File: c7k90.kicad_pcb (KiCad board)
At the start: 2 copper layers, 71.5 x 27.1 mm, 5 parts, among them J1 Conn_01x02_Socket, J2 Conn_01x04_Socket, J3 Conn_01x04_Pin, SW1 SW_SPST, U1 Nice! Nano (ProMicro)

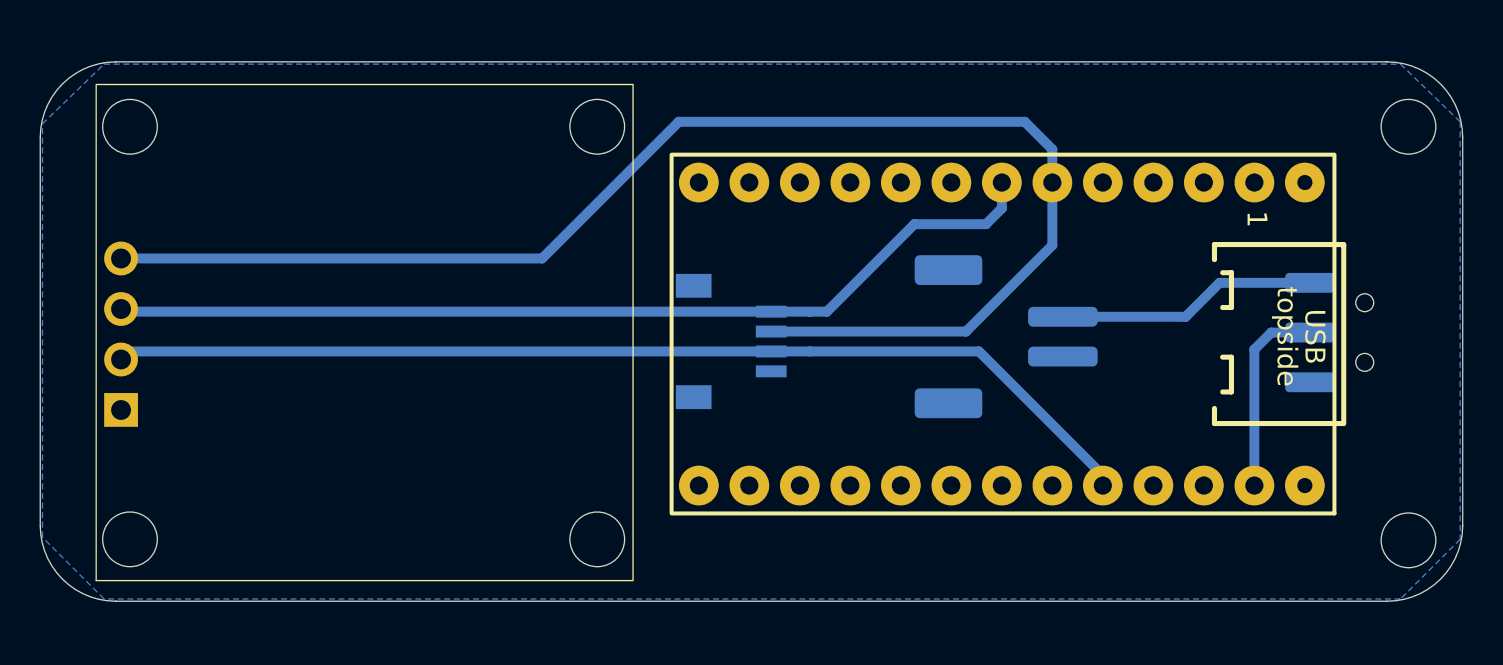
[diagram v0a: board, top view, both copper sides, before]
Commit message: updates
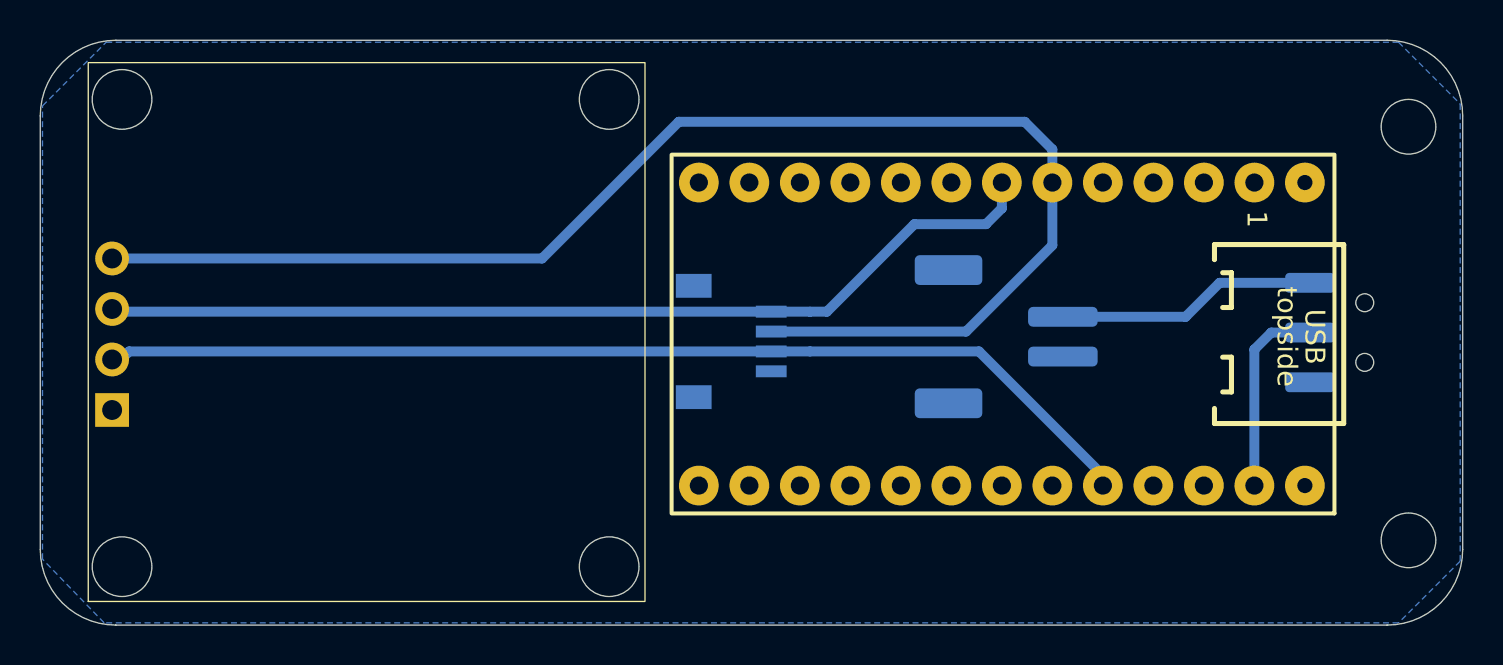
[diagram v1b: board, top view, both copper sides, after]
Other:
- board size 71.5 x 27.1 mm -> 71.5 x 29.4 mm
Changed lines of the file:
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@@
 		(attr through_hole)
 		(fp_rect
-			(start -12.45 -12)
-			(end 12.5 15)
+			(start -13.5 -12.4)
+			(end 13.6 15.6)
 			(stroke
 				(width 0.05)
@@
 		)
 		(fp_circle
-			(center 10.375 -10.3)
-			(end 10.375 -11.675)
+			(center 11.75 -10.7)
+			(end 13.25 -10.7)
 			(stroke
 				(width 0.05)
@@
 		)
 		(fp_circle
-			(center -10.375 -10.3)
-			(end -10.375 -11.675)
+			(center -11.75 -10.7)
+			(end -10.25 -10.7)
 			(stroke
 				(width 0.05)
@@
 		)
 		(fp_circle
-			(center 10.375 13.2)
-			(end 11.75 13.2)
+			(center 11.75 13.8)
+			(end 13.25 13.8)
 			(stroke
 				(width 0.05)
@@
 		)
 		(fp_circle
-			(center -10.375 13.2)
-			(end -9 13.2)
+			(center -11.75 13.8)
+			(end -10.25 13.8)
 			(stroke
 				(width 0.05)
@@
 		)
 		(pad "1" thru_hole rect
-			(at -3.87 -10.75 90)
+			(at -3.87 -11.2 90)
 			(size 1.7 1.7)
 			(drill 1)
@@
 		)
 		(pad "2" thru_hole circle
-			(at -1.33 -10.75 90)
+			(at -1.33 -11.2 90)
 			(size 1.7 1.7)
 			(drill 1)
@@
 		)
 		(pad "3" thru_hole circle
-			(at 1.21 -10.75 90)
+			(at 1.21 -11.2 90)
 			(size 1.7 1.7)
 			(drill 1)
@@
 		)
 		(pad "4" thru_hole circle
-			(at 3.75 -10.75 90)
+			(at 3.75 -11.2 90)
 			(size 1.7 1.7)
 			(drill 1)
@@
 		)
 		(embedded_fonts no)
-		(model "/Users/sklarm/Documents/KiCad/mikeysklar/3dmodels/oled-ssd1306.step"
+		(model "/Users/sklarm/Documents/KiCad/mikeysklar/3dmodels/blue-oled-ssd1306-128x64.step"
 			(offset
-				(xyz 0 -1 0)
+				(xyz 0 -1.5 0)
 			)
 			(scale
@@
 	)
 	(gr_line
-		(start 209.125988 72.987007)
-		(end 145.187006 72.987006)
+		(start 209.125988 71.900001)
+		(end 145.187006 71.9)
 		(stroke
 			(width 0.05)
@@
 	)
 	(gr_arc
-		(start 212.925988 96.312994)
-		(mid 211.812994 99)
-		(end 209.125988 100.112994)
+		(start 212.925988 97.512994)
+		(mid 211.812994 100.2)
+		(end 209.125988 101.312994)
 		(stroke
 			(width 0.05)
@@
 	)
 	(gr_arc
-		(start 209.125988 72.987006)
-		(mid 211.812994 74.1)
-		(end 212.925988 76.787006)
+		(start 209.125988 71.9)
+		(mid 211.812999 73.01299)
+		(end 212.925988 75.7)
 		(stroke
 			(width 0.05)
@@
 	)
 	(gr_line
-		(start 212.925988 96.312994)
-		(end 212.925988 76.787006)
+		(start 212.925988 97.512994)
+		(end 212.925988 75.709549)
 		(stroke
 			(width 0.05)
@@
 	)
 	(gr_line
-		(start 141.387006 76.787006)
-		(end 141.387006 96.312994)
+		(start 141.387006 75.7)
+		(end 141.387006 97.512994)
 		(stroke
 			(width 0.05)
@@
 	)
 	(gr_arc
-		(start 145.187006 100.112994)
-		(mid 142.5 99)
-		(end 141.387006 96.312994)
+		(start 145.187006 101.312994)
+		(mid 142.5 100.2)
+		(end 141.387006 97.512994)
 		(stroke
 			(width 0.05)
@@
 	)
 	(gr_line
-		(start 209.125988 100.112987)
-		(end 145.187 100.112992)
+		(start 209.125988 101.312987)
+		(end 145.187 101.312992)
 		(stroke
 			(width 0.05)
@@
 	)
 	(gr_arc
-		(start 141.387006 76.787006)
-		(mid 142.5 74.1)
-		(end 145.187006 72.987006)
+		(start 141.387006 75.7)
+		(mid 142.5 73.012994)
+		(end 145.187006 71.9)
 		(stroke
 			(width 0.05)
@@
 		(polygon
 			(pts
-				(xy 144.6 73.1) (xy 209.8 73.1) (xy 212.8 76) (xy 212.8 97) (xy 209.8 100) (xy 144.6 100) (xy 141.5 96.9)
-				(xy 141.5 76.1)
-			)
-		)
+				(xy 144.7 72) (xy 209.7 72) (xy 212.8 75.1) (xy 212.8 98.1) (xy 209.7 101.2) (xy 144.6 101.2) (xy 141.5 98)
+				(xy 141.5 75.2)
+			)
+		)
